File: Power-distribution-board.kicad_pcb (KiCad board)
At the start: 4 copper layers, 128.3 x 105.4 mm, 89 parts, among them J10 2606-1104/020-000, J11 178.6165.0001, J12 2606-1104/020-000, J13 2606-1104/020-000, J14 178.6165.0001, J15 2606-1104/020-000, J16 2606-1104/020-000, J17 178.6165.0001, J18 178.6165.0001, J19 178.6165.0001, J7 Screw_Terminal_01x03, J8 178.6165.0001, J9 USB_C_Receptacle_USB2.0_14P, SW1 SW_Nidec_CAS-120A1, U1 ESP32-S3-WROOM-1, U11 TJA1051TK-3, U12 INA220BIDGSR, U13 INA220BIDGSR, U14 INA220BIDGSR, U15 INA220BIDGSR, U16 INA220BIDGSR, U17 INA220BIDGSR, U18 CP2102N-Axx-xQFN24, U2 LM3940IT-3.3, U3 INA220BIDGSR, U4 LM317_SOT-223, U5 TM1637, U6 CC56-12EWA

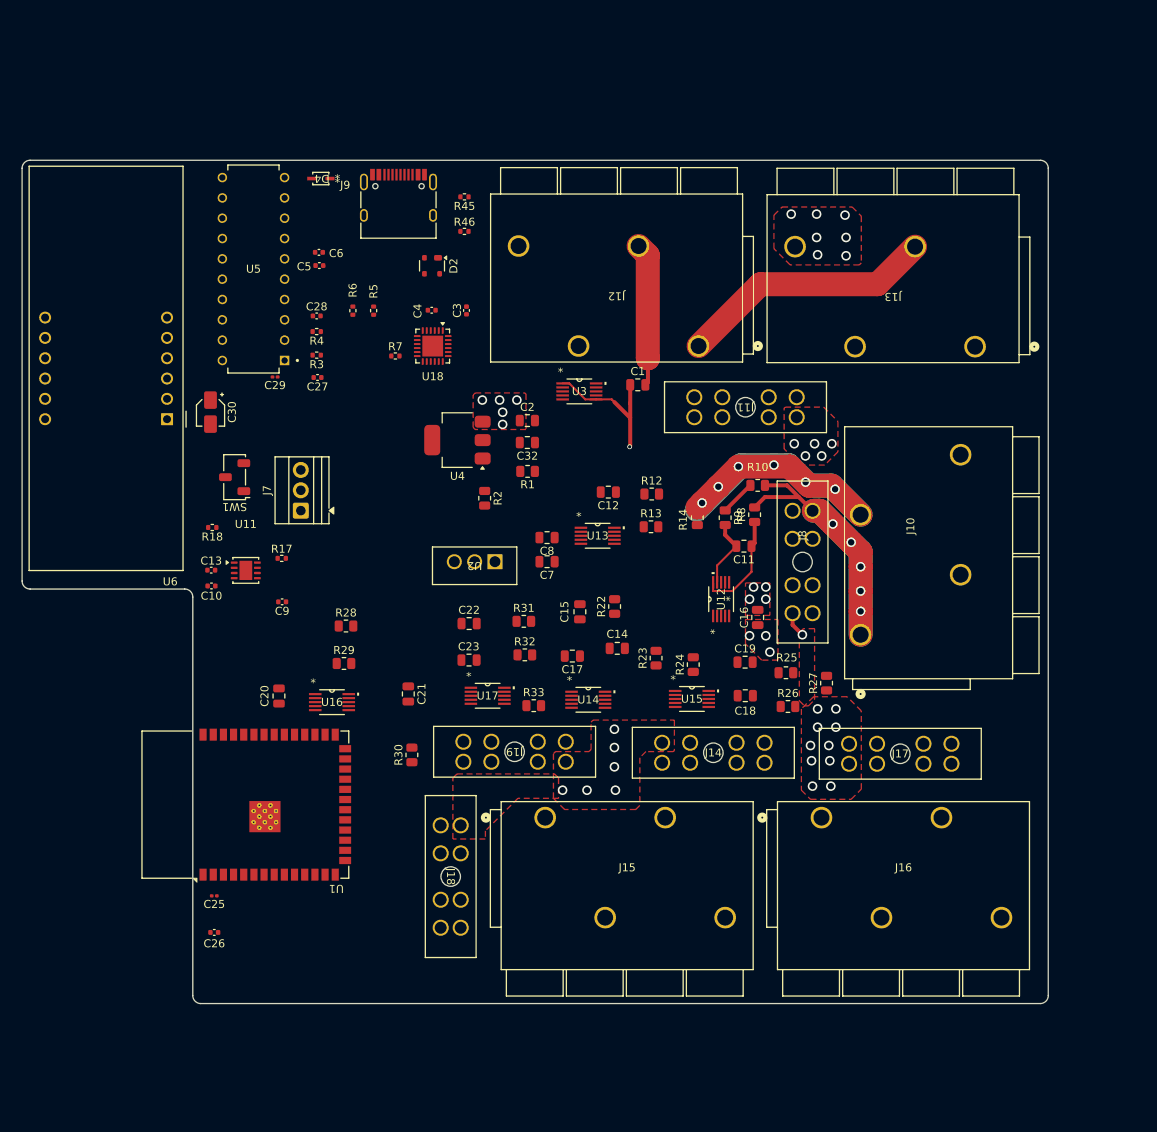
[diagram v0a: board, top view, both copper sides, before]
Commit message: cleaned up repo
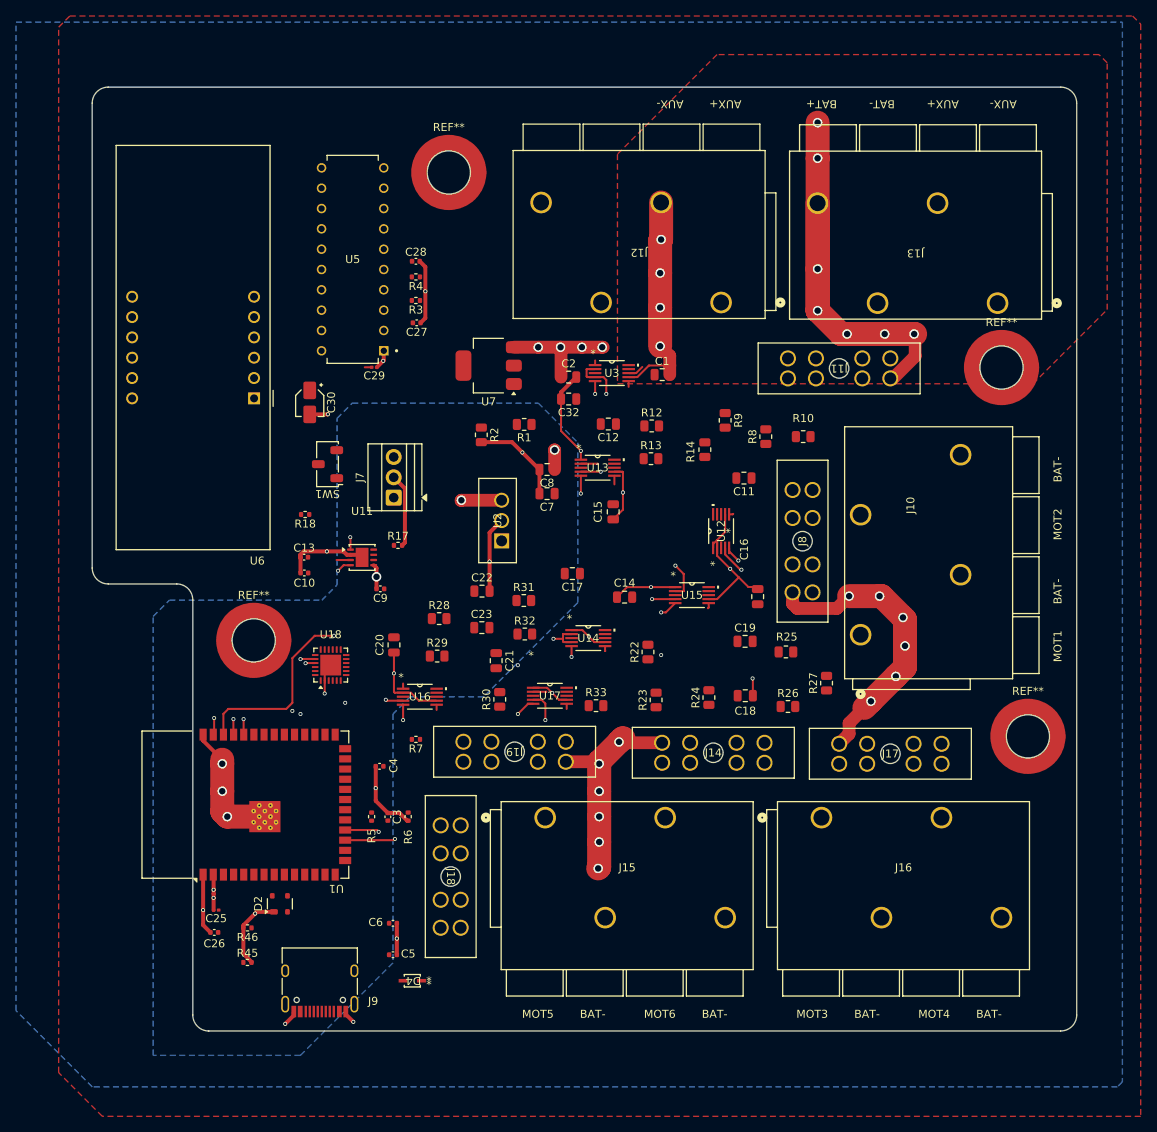
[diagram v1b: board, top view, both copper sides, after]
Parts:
- removed U4: LM317_SOT-223, Package_TO_SOT_SMD:SOT-223-3_TabPin2
- added REF**: Mounting_Wuerth_WA-SMST-4.5mm_H1mm_9774010982, Mounting_Wuerth:Mounting_Wuerth_WA-SMST-4.5mm_H1mm_9774010982, F.Cu at (243.3, 74.2)
- added REF**: Mounting_Wuerth_WA-SMST-4.5mm_H1mm_9774010982, Mounting_Wuerth:Mounting_Wuerth_WA-SMST-4.5mm_H1mm_9774010982, F.Cu at (246.6, 120.3)
- added REF**: Mounting_Wuerth_WA-SMST-4.5mm_H1mm_9774010982, Mounting_Wuerth:Mounting_Wuerth_WA-SMST-4.5mm_H1mm_9774010982, F.Cu at (149.9, 108.3)
- added REF**: Mounting_Wuerth_WA-SMST-4.5mm_H1mm_9774010982, Mounting_Wuerth:Mounting_Wuerth_WA-SMST-4.5mm_H1mm_9774010982, F.Cu at (174.2, 49.8)
- added U7: LM317_SOT-223, Package_TO_SOT_SMD:SOT-223-3_TabPin2, F.Cu at (179.2, 73.9)
- moved D4 100.9 mm to (169.7, 150.8)
- moved R45 99.5 mm to (149.1, 148.5), turned to 0 degrees
- moved J9 97.0 mm to (158.1, 150.6), turned to 180 degrees
- moved R46 91.2 mm to (149.1, 144.2), turned to 180 degrees
- moved C5 86.6 mm to (167.3, 147.6), turned to 0 degrees
- moved C6 84.4 mm to (167.3, 143.6), turned to 0 degrees
- moved D2 82.0 mm to (153.1, 141.2), turned to 90 degrees
- moved C3 64.1 mm to (166.6, 130.3), turned to -90 degrees
- moved R6 63.6 mm to (169.2, 130.3), turned to -90 degrees
- moved R5 63.3 mm to (164.6, 130.3), turned to -90 degrees
- moved C4 57.4 mm to (165.6, 124.0), turned to 0 degrees
- moved R7 48.0 mm to (170.1, 120.7), turned to 180 degrees
- moved U18 41.9 mm to (159.5, 111.4), turned to 90 degrees
- moved C20 15.7 mm to (167.4, 108.8)
- moved R17 14.6 mm to (167.9, 96.4)
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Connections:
- J10 pad 2: GND -> /BATN
- J10 pad 4: GND -> /BATN
- J13 pad 3: GND -> /BATN
- J15 pad 2: GND -> /BATN
- J15 pad 4: GND -> /BATN
- J16 pad 2: GND -> /BATN
- J16 pad 4: GND -> /BATN
- U17 pad 1: unconnected-(U17-A1-Pad1) -> GND
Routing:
- net GND: track 0.01 -> 176.6 mm, vias 4 -> 24
- net /SDA: track 0.00 -> 148.6 mm, vias 0 -> 8
- net /SCL: track 0.00 -> 140.2 mm, vias 0 -> 11
- net /BATP: track 3.31 -> 135.7 mm, vias 34 -> 23
- net /MOT2: track 50.4 -> 0.00 mm, vias 6 -> 0
- net /MOT1: track 50.0 -> 0.00 mm, vias 5 -> 0
- net /CAN TX: track 0.00 -> 41.8 mm, vias 0 -> 3
- net /CAN RX: track 0.00 -> 33.9 mm, vias 0 -> 2
- net /AUX+: track 32.2 -> 2.02 mm
- net /UART TX: track 0.00 -> 18.5 mm, vias 0 -> 3
- net /UART RX: track 0.00 -> 17.3 mm, vias 0 -> 3
- net /3.3V: track 0.00 -> 15.1 mm, vias 0 -> 5
- net Net-(U12-VIN+): track 13.4 -> 0.00 mm
- net /AUX-: track 18.0 -> 27.8 mm, vias 0 -> 4
- net Net-(U12-VIN-): track 8.75 -> 0.00 mm
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- added copper zone on B.Cu, net /3.3V
- added copper zone on F.Cu, net /AUX+
- added copper zone on In2.Cu, net /AUX-
- added copper zone on In1.Cu, net /BATN
- added copper zone on B.Cu, net /BATP
- added copper zone on In2.Cu, net GND
- removed copper zone on In2.Cu, net /3.3V
- removed copper zone on In2.Cu, net /5V
- removed copper zone on F.Cu, net /BATP
- removed copper zone on In2.Cu, net /BATP
- removed copper zone on F.Cu, net GND
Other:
- board size 128.3 x 105.4 mm -> 123.1 x 118 mm
- board text added: "AUX+"
- board text added: "AUX-"
- board text added: "BAT+"
- board text added: "BAT-"
- board text added: "MOT1"
- board text added: "MOT2"
- board text added: "MOT3"
- board text added: "MOT4"
- board text added: "MOT5"
- board text added: "MOT6"
